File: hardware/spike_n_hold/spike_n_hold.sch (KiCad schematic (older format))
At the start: 59 parts, among them J1 input_trigger_2, J2 input_trigger_1, J3 to_solenoid_2, J4 to_solenoid_1, J5 Conn_01x02, J6 Conn_01x02, Q1 MJH11021G, Q2 MJH11021G, Q3 MPSA42, Q4 MPSA42, Q5 MPSA42, Q6 MPSA42, Q7 MJH11022G, Q8 MJH11022G, Q9 IRFZ24NPBF, U1 LM555xM, U2 LM555xM, U3 LM555xM

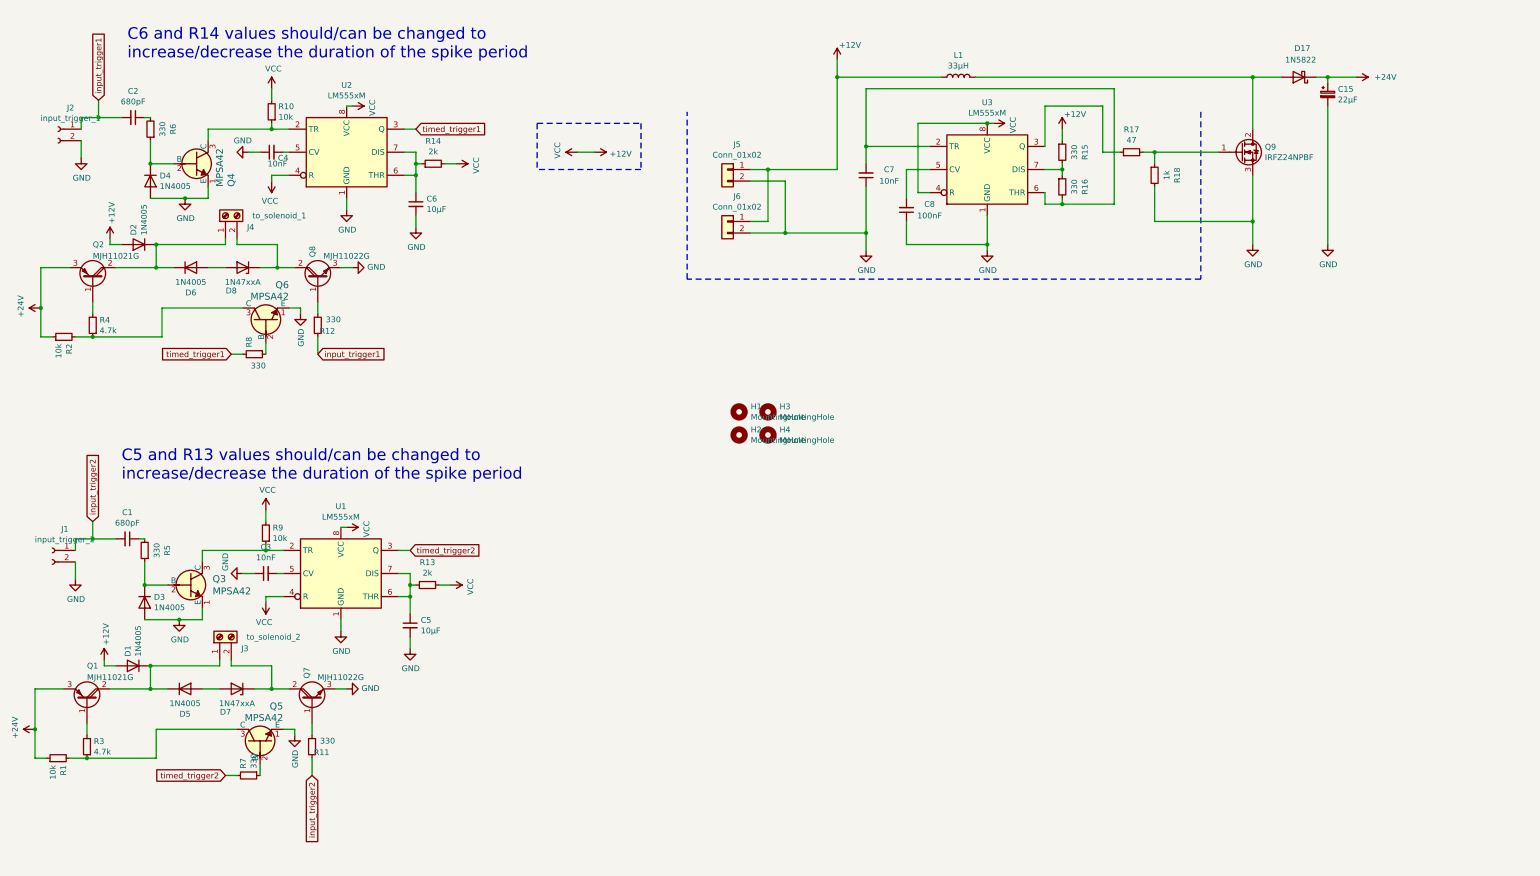
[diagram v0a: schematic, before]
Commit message: Update board and add gerbers
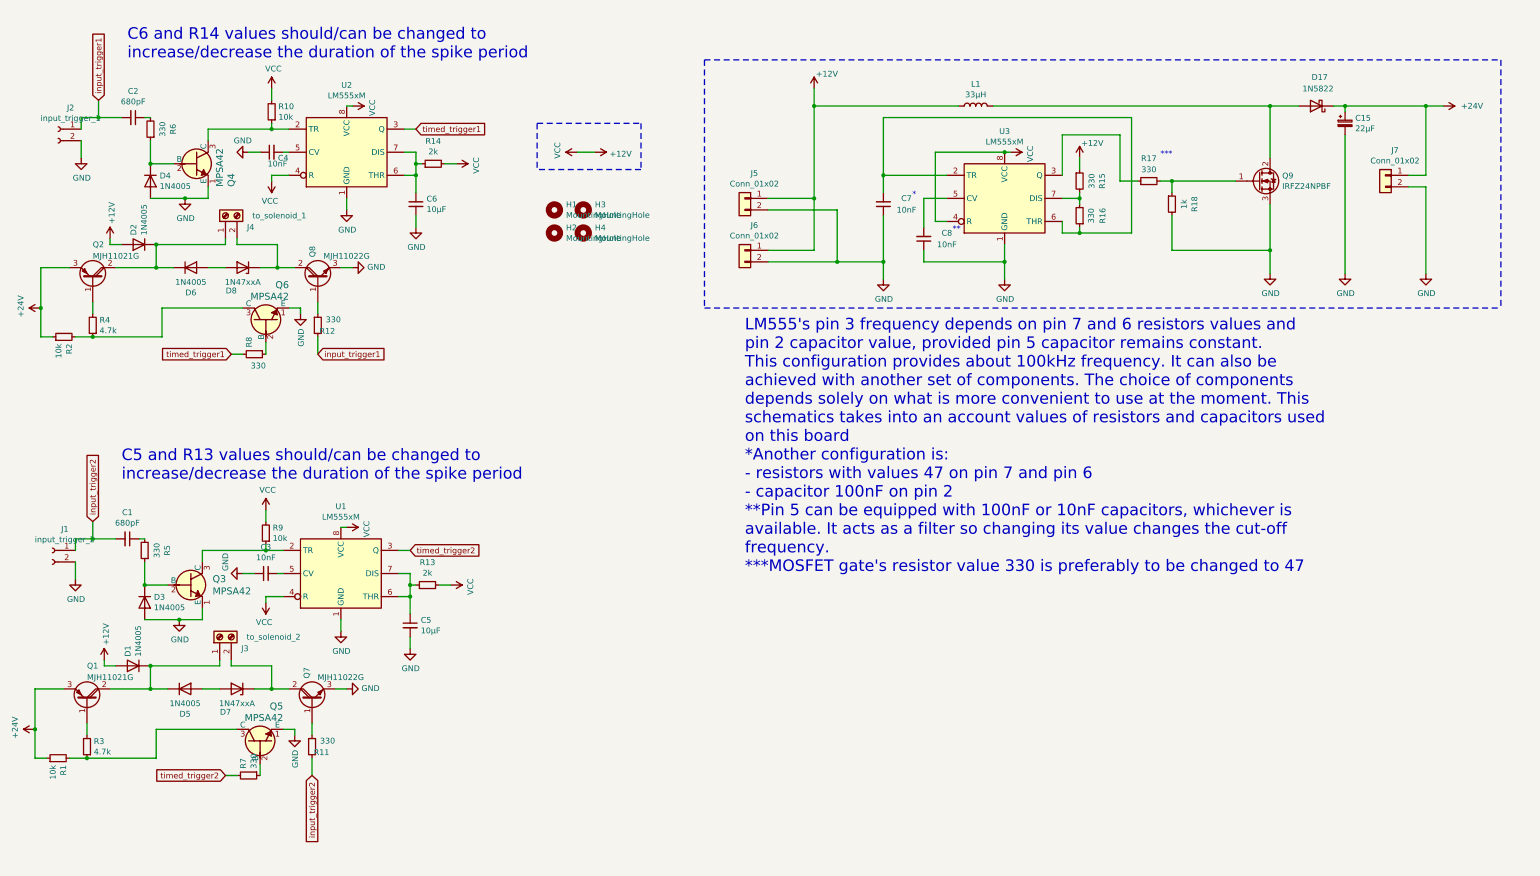
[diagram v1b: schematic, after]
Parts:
- added J7: Conn_01x02, Connector_JST:JST_XH_B2B-XH-A_1x02_P2.50mm_Vertical, symbol Connector_Generic:Conn_01x02
- C8: value 100nF -> 10nF
- R17: value 47 -> 330
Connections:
- net +24V: now also J7.1 (Pin_1)
- net GND: now also J7.2 (Pin_2)
- net at R15.2, U3.7 (DIS): now also R16.2; no longer R16.1
- net at C7.2, U3.2 (TR), U3.6 (THR): now also R16.1; no longer R16.2
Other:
- note added: "*"
- note added: "**"
- note added: "***"
- note added: "LM555's pin 3 frequency depends on pin 7 and 6 resistors values and\npin 2 capacitor value, provided pin 5 capacitor remains constant.\nThis configuration provides about 100kHz frequency. It can also be\nachieved with another set of components. The choice of components\ndepends solely on what is more convenient to use at the moment. This \nschematics takes into an account values of resistors and 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"
- moved on the sheet: C15, C7, C8, D17, H1, H2, H3, H4, J5, J6, L1, Q9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
